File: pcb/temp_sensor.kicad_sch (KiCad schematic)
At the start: 3 parts, among them U6 LM75ADP

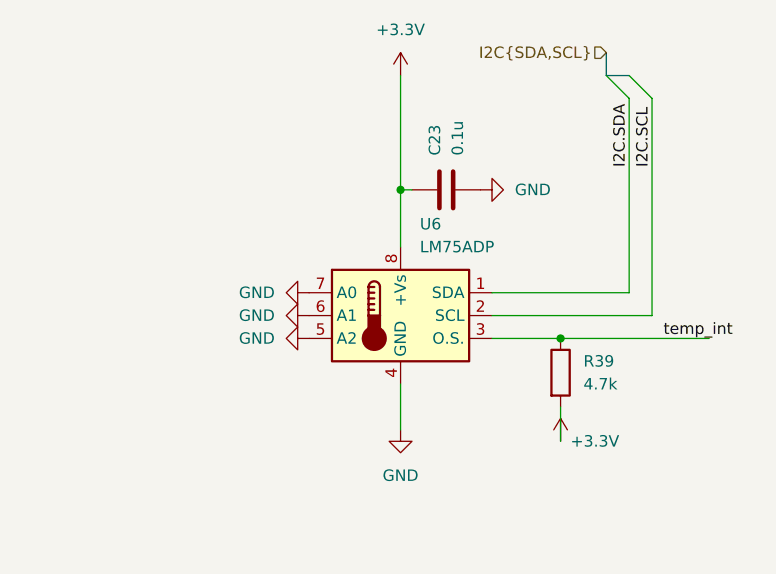
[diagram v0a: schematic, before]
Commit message: cleanup routing
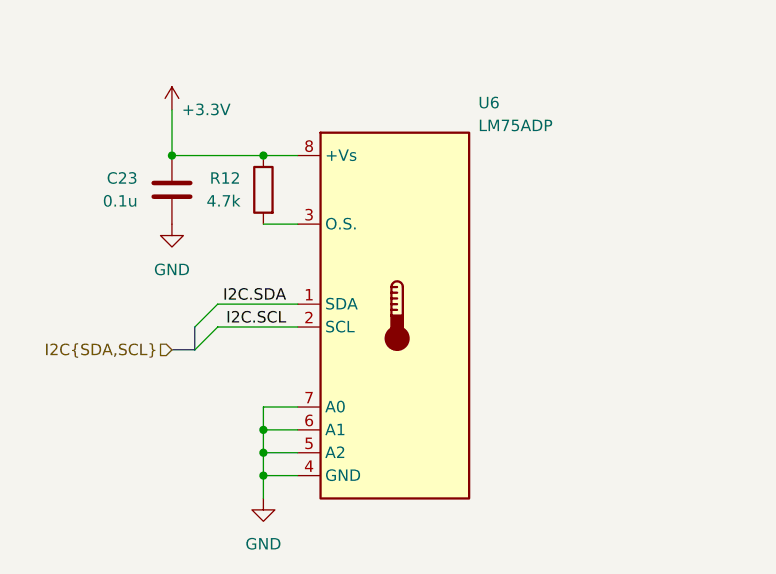
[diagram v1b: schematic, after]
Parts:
- removed R39: 4.7k, symbol Device:R
- added R12: 4.7k, symbol Device:R
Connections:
- net +3.3V: now also R12.1
- net temp_int: no longer names the net of U6.3 (O.S.)
- net temp_int: now also R12.2
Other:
- moved on the sheet: U6
